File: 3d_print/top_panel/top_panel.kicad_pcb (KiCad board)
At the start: 2 copper layers, 90 x 40 mm, 22 parts

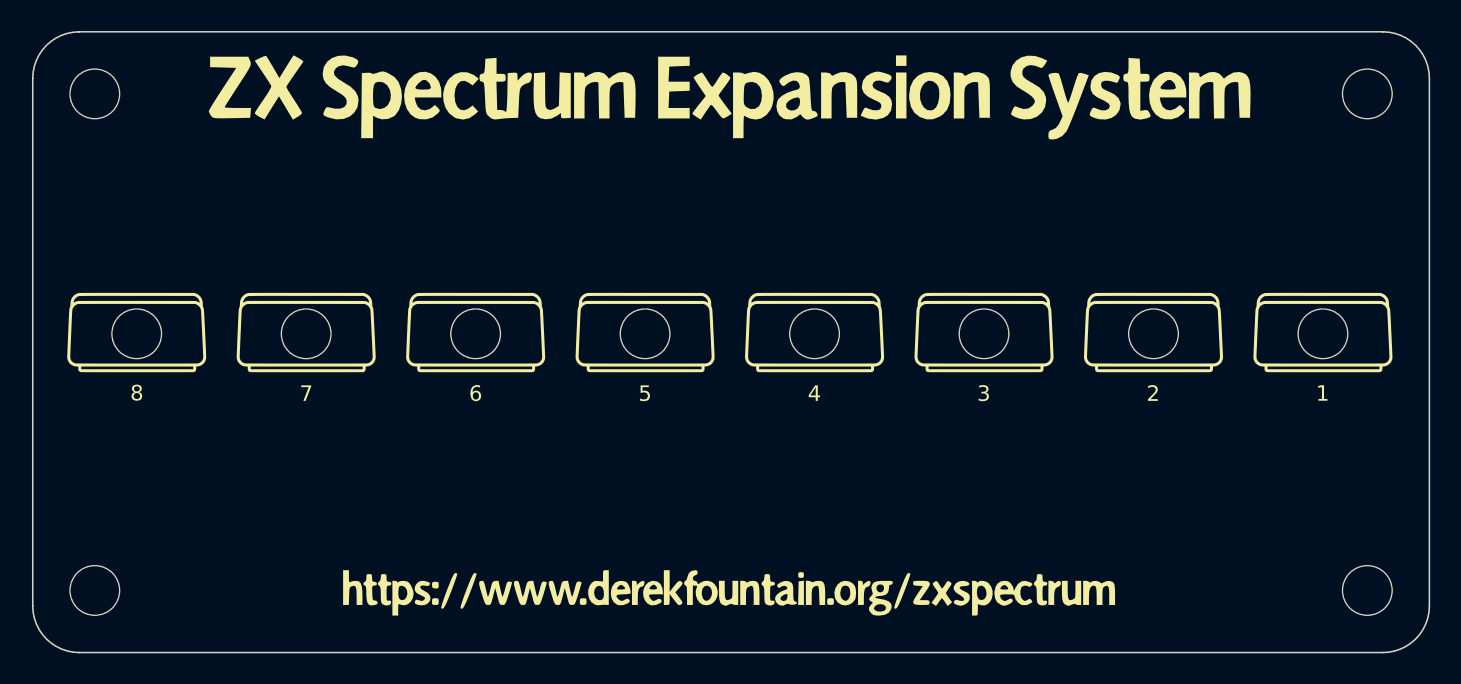
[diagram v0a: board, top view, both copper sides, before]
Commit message: lots more work to finalise the board pre-fab
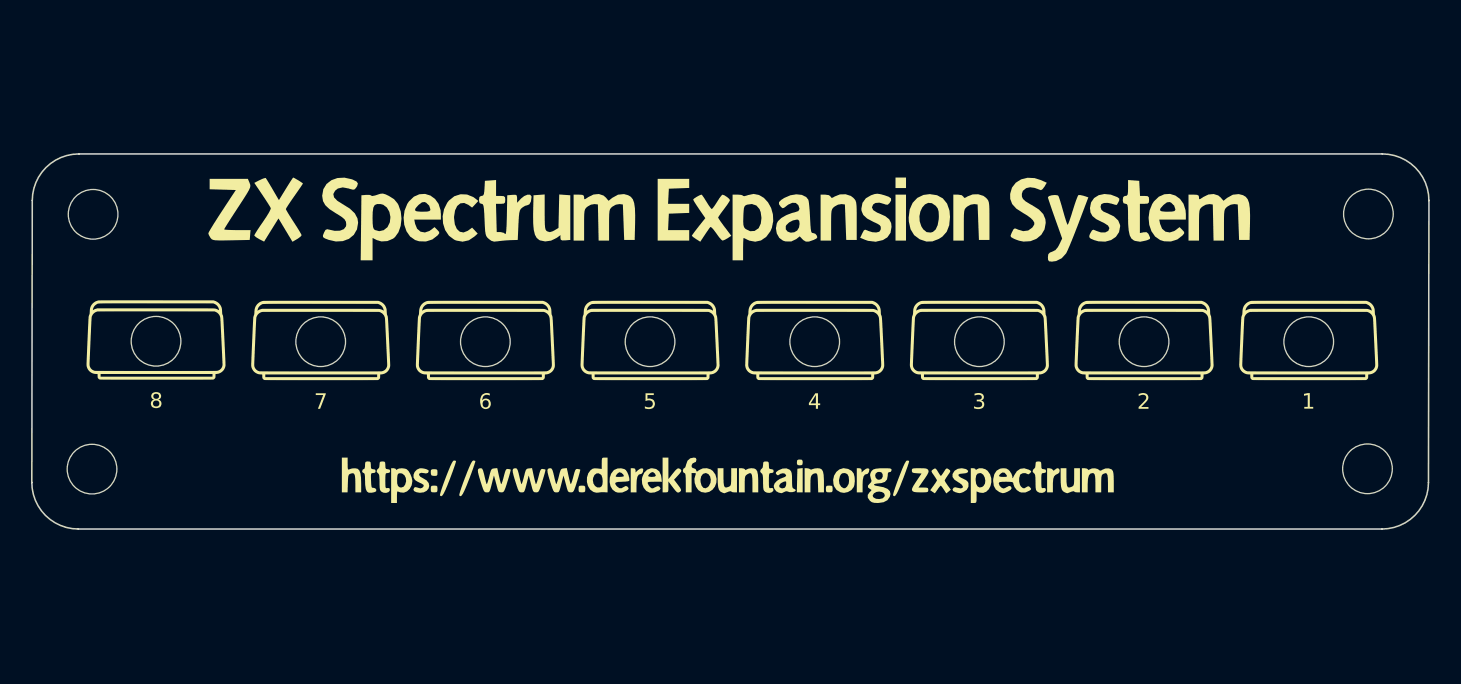
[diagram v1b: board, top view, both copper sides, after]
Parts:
- moved G*** 7.87 mm to (144.7, 71.7)
- moved REF** 7.84 mm to (186.0, 88.2)
- moved REF** 7.82 mm to (103.8, 88.2)
- moved REF** 7.76 mm to (103.9, 71.8)
- moved REF** 7.74 mm to (186.1, 71.7)
- moved G*** 7.26 mm to (144.8, 88.7)
- moved ? 1.33 mm to (107.9, 79.9)
- moved G*** 1.33 mm to (107.9, 79.9)
- moved ? 1.07 mm to (118.6, 80.0)
- moved G*** 1.07 mm to (118.6, 79.9)
- moved ? 1.05 mm to (182.2, 80.0)
- moved G*** 1.05 mm to (182.2, 79.9)
- moved ? 0.81 mm to (129.2, 80.0)
- moved G*** 0.81 mm to (129.2, 79.9)
- moved ? 0.79 mm to (171.6, 80.0)
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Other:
- board size 90 x 40 mm -> 90 x 24.2 mm
